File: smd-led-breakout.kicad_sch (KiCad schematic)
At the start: 15 parts

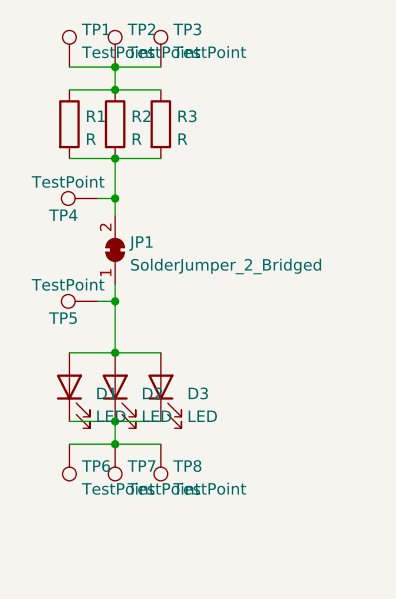
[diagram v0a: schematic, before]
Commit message: Refinements
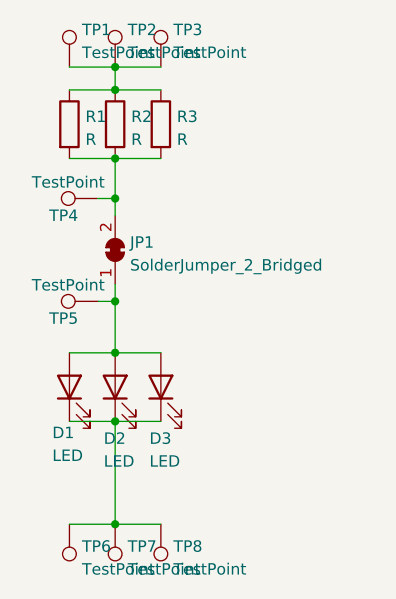
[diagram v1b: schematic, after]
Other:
- moved on the sheet: TP6, TP7, TP8
